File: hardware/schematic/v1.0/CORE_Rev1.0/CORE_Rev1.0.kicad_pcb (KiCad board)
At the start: 4 copper layers, 102.6 x 102.3 mm, 122 parts, among them CN1 LAIL-PHC2_54-2P-01-XH-L, J1 Conn_01x06_Socket, J10 USB_C_Receptacle_USB2.0_16P, J11 Conn_01x06_Socket, J12 USB_C_Receptacle_USB2.0_16P, J13 Conn_01x04_Socket, J14 Conn_01x03_Socket, J15 Conn_01x05_Socket, J16 Conn_01x04_Socket, J26 Conn_01x04_Socket, M1 ZYNQ7010&7020, Q1 Si2302CDS-T1-GE3, U1 TXS02612RTWR, U10 IPEX1, U11 IPEX1, U12 FT2232HL, U13 IPEX1, U14 IPEX1, U15 IPEX1, U16 IPEX1, U17 IPEX1, U18 IPEX1, U19 IPEX1, U2 TPS78633, U20 IPEX1, U21 IPEX1, U22 IPEX1, U23 IPEX1, U24 IPEX1, U25 IPEX1, U26 IPEX1, U27 IPEX1, U28 IPEX1, U3 SD_Card, U4 IPEX1, U5 AMS1117-1.8, U6 93LC56BT-I_OT, U7 FPC-6P, U8 IPEX1, U9 IPEX1, X1 X322512MSB4SI

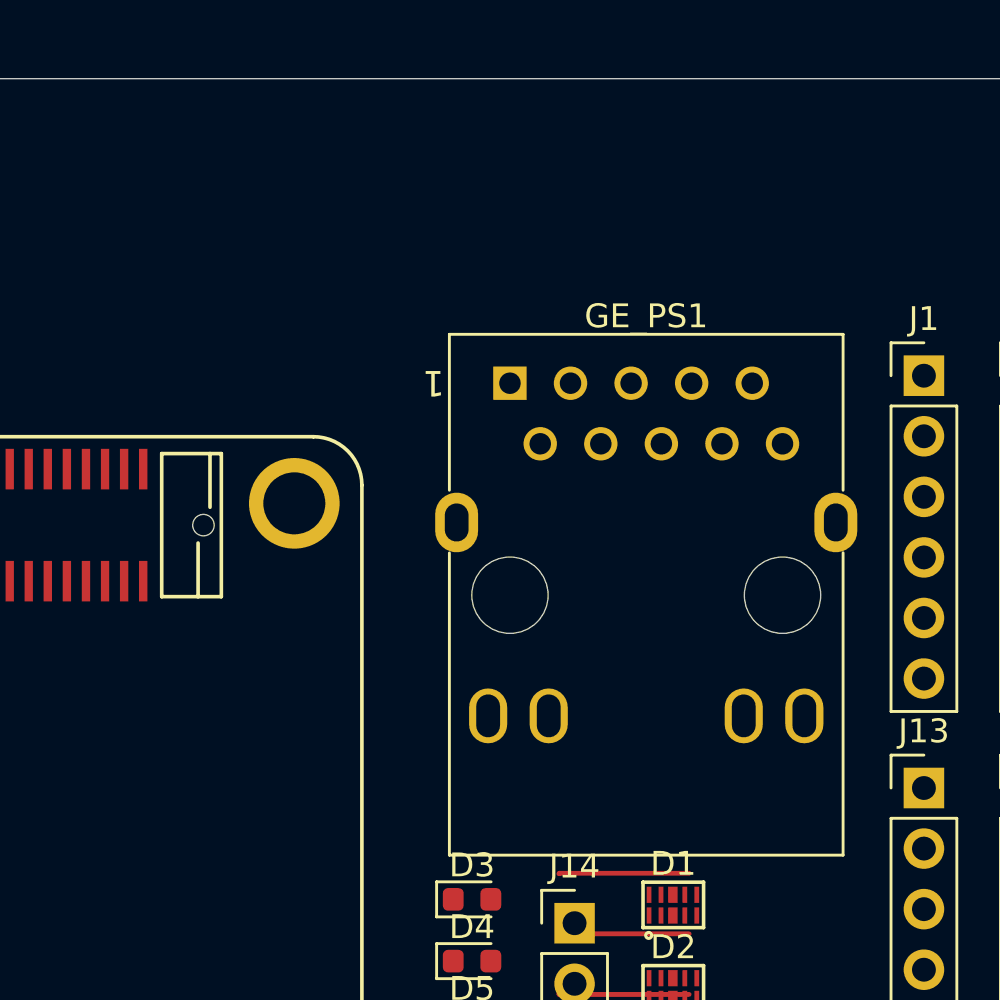
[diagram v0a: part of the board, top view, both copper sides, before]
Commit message: sch update
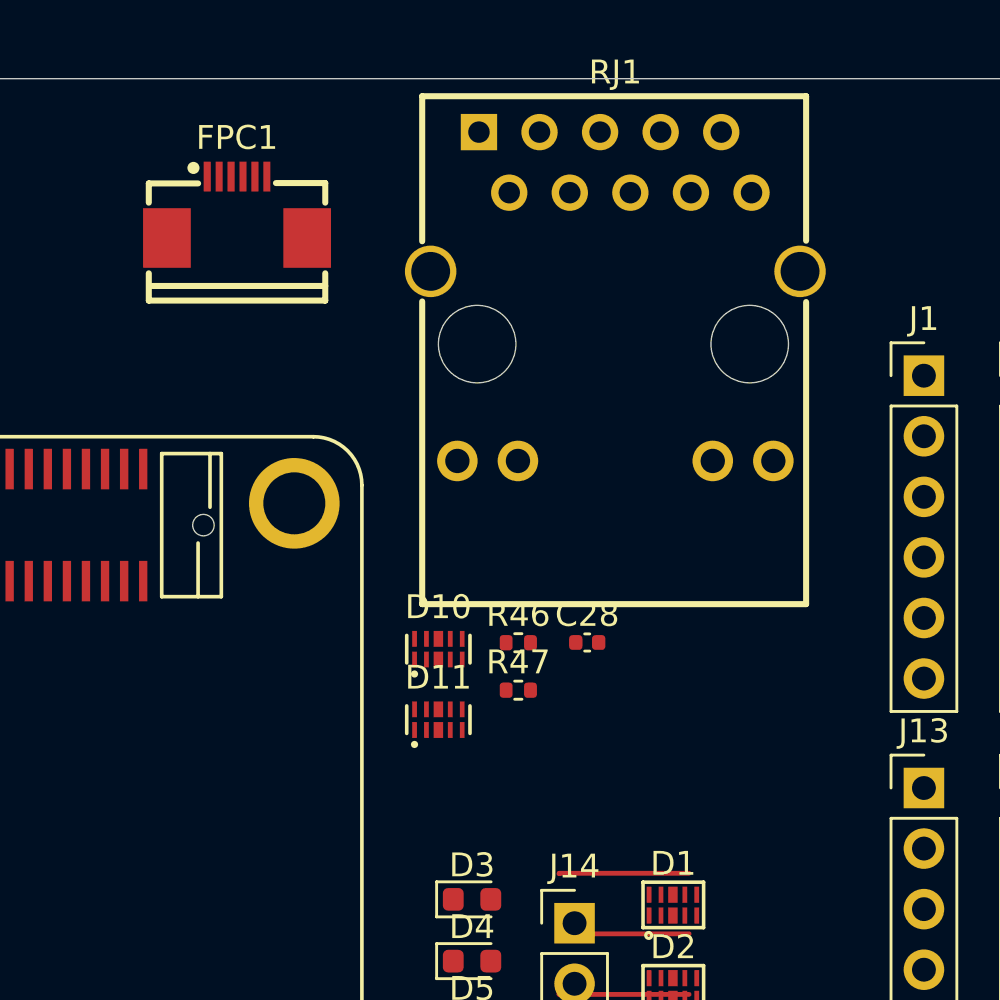
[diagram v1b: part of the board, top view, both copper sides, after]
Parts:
- removed GE_PS1: HR911131A, Counter:HR911131A
- added C28: 100nF, Capacitor_SMD:C_0402_1005Metric, F.Cu at (178.9, 72.5)
- added D10: AZ1143-04F_R7G, CORE:AZ1143-04F_R7G, F.Cu at (172.6, 72.8)
- added D11: AZ1143-04F_R7G, CORE:AZ1143-04F_R7G, F.Cu at (172.6, 75.8)
- added FPC1: FPC-05F-6PH20, CORE:FPC-05F-6PH20, F.Cu at (164.2, 54.3)
- added R46: 499R, Resistor_SMD:R_0402_1005Metric, F.Cu at (176.0, 72.5)
- added R47: 499R, Resistor_SMD:R_0402_1005Metric, F.Cu at (176.0, 74.5)
- added RJ1: HR911131A, CORE:HR911131A, F.Cu at (180.1, 58.0)
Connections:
- C1 pad 1: Net-(GE_PS1-CT1) -> GND
- C1 pad 2: GND -> Net-(C1-Pad2)
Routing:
- net GND: track 0.00 -> 5.46 mm
- net (no net): track 16.4 -> 10.9 mm

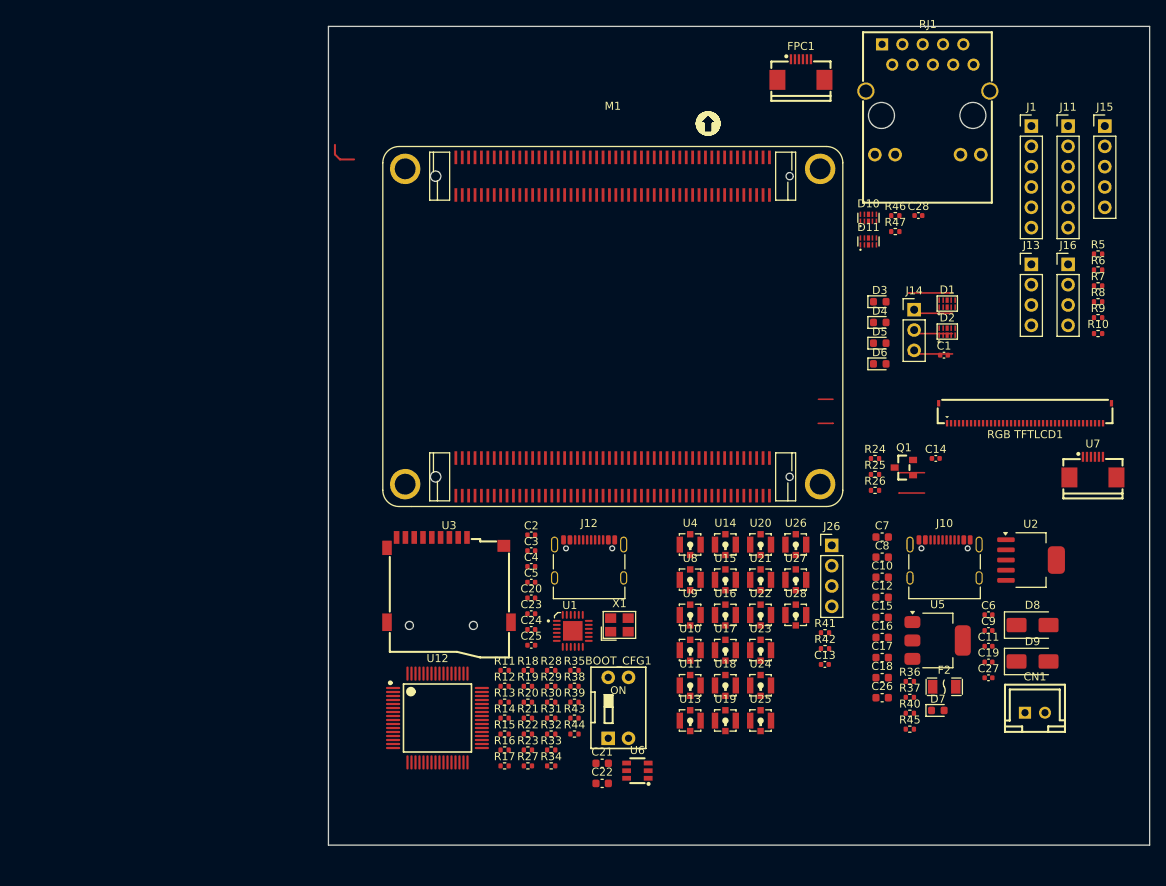
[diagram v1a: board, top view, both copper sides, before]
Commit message: sch update
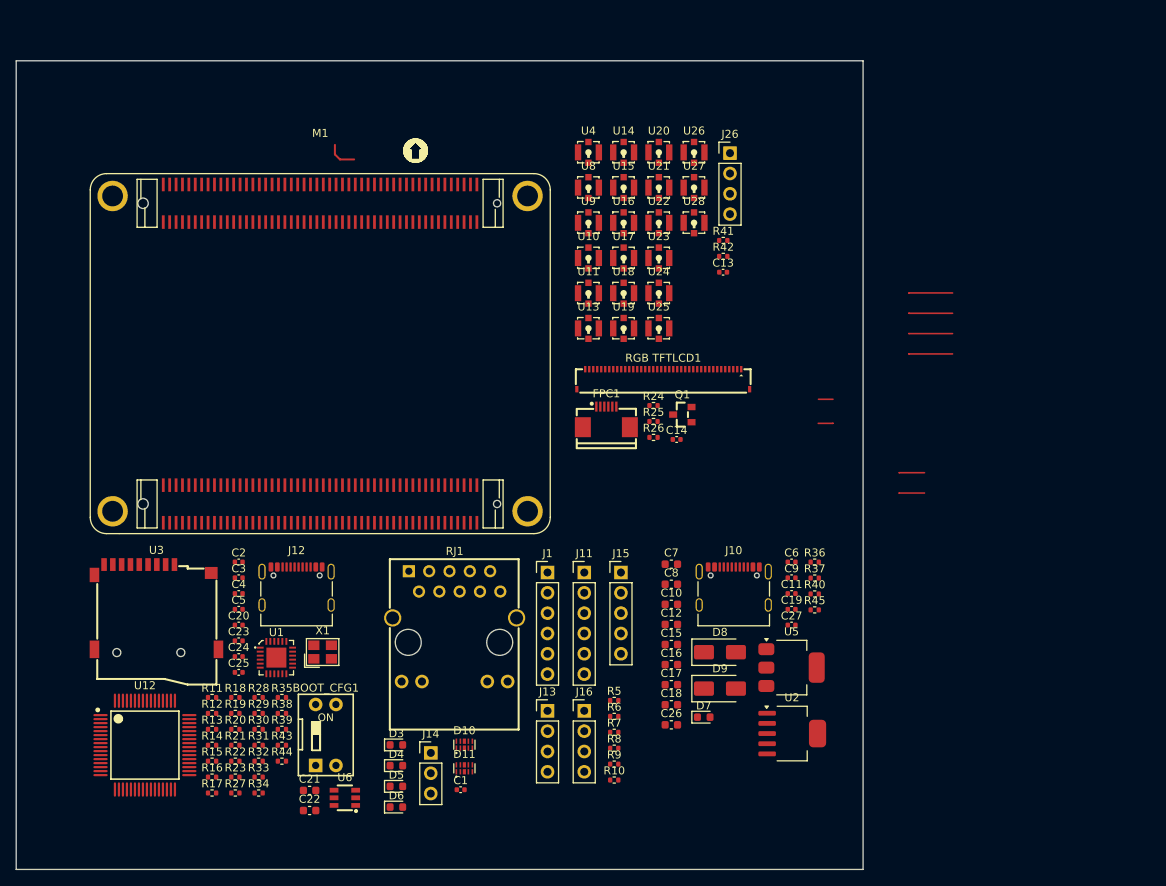
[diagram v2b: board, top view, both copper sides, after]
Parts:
- removed C28: 100nF, Capacitor_SMD:C_0402_1005Metric
- removed CN1: LAIL-PHC2_54-2P-01-XH-L, JLCImport:LAIL-PHC2_54-2P-01-XH-L
- removed D1, D2: AZ1143-04F.R7G, Counter:DFN2510P10E
- removed F2: BSMD1206C-1300T, JLCImport:BSMD1206C-1300T
- removed R46, R47: 499R, Resistor_SMD:R_0402_1005Metric
- removed U7: FPC-6P, CORE:FPC-05F-6PH20
- U1: footprint Counter:QFN24_RTW -> CORE:TXS02612RTWR
- U3: footprint Counter:SIM-SMD_LX_XDFP-0090-012 -> CORE:XDFP-0090-012
- moved RJ1 88.5 mm to (120.9, 123.9)
- moved D10 83.0 mm to (122.1, 138.7)
- moved D11 83.0 mm to (122.1, 141.6)
- moved R5 82.3 mm to (140.9, 133.1)
- moved J1 82.3 mm to (132.5, 117.2)
- moved J11 82.3 mm to (137.1, 117.2)
- moved J13 82.3 mm to (132.5, 134.4)
- moved J15 82.3 mm to (141.7, 117.2)
- moved J16 82.3 mm to (137.1, 134.4)
- moved R10 82.3 mm to (140.9, 143.1)
- moved R6 82.3 mm to (140.9, 135.1)
- moved R7 82.3 mm to (140.9, 137.1)
- moved R8 82.3 mm to (140.9, 139.1)
- moved R9 82.3 mm to (140.9, 141.1)
- moved D3 82.0 mm to (113.6, 138.7)
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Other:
- board size 102.6 x 102.3 mm -> 105.9 x 101.1 mm
